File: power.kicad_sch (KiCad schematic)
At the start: 24 parts, among them J1 USB_C_Receptacle_USB2.0_14P, J8 Conn_01x04, J9 Conn_01x04, U4 TPS6282x

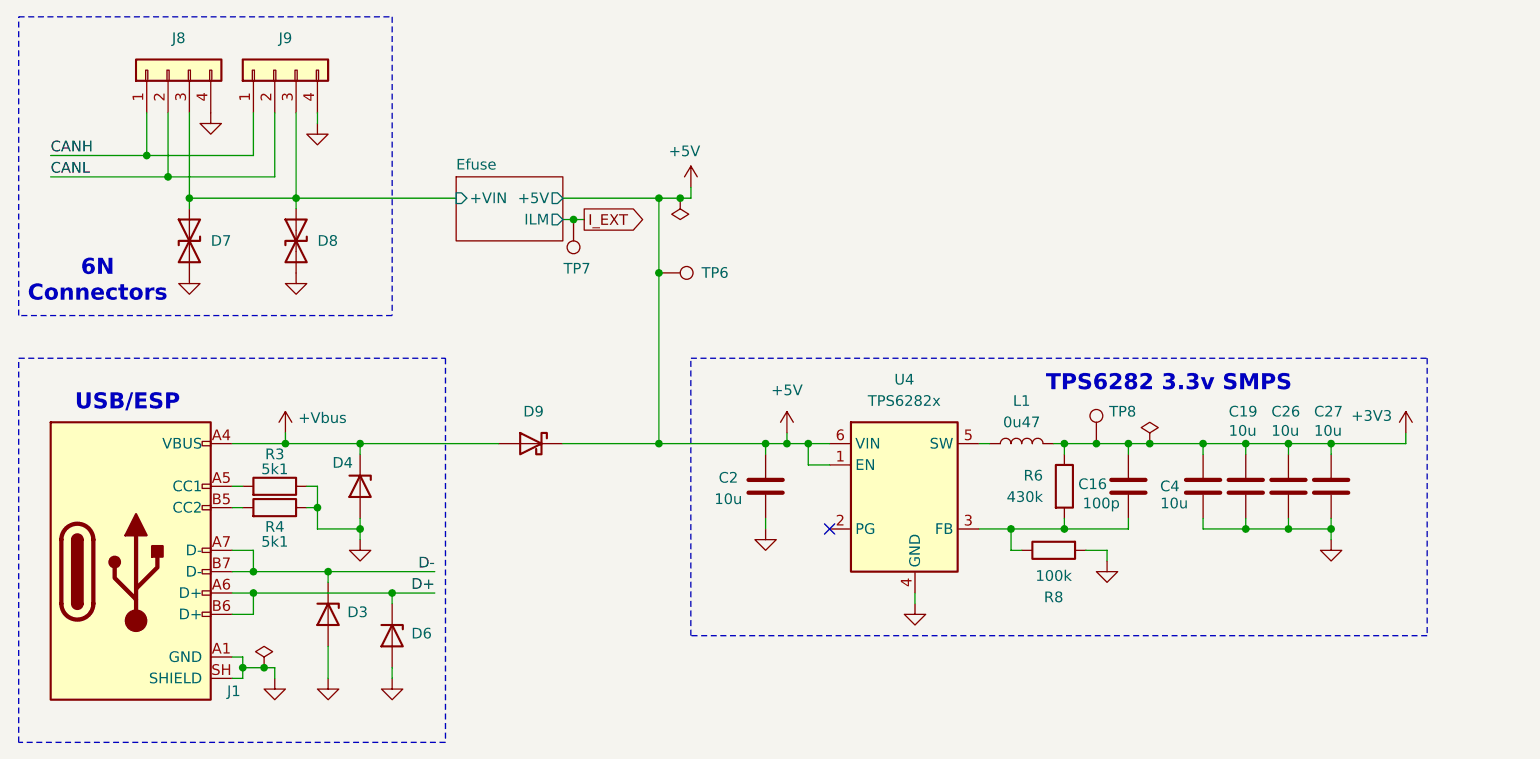
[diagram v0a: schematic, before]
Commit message: schem: add +3v8 smps
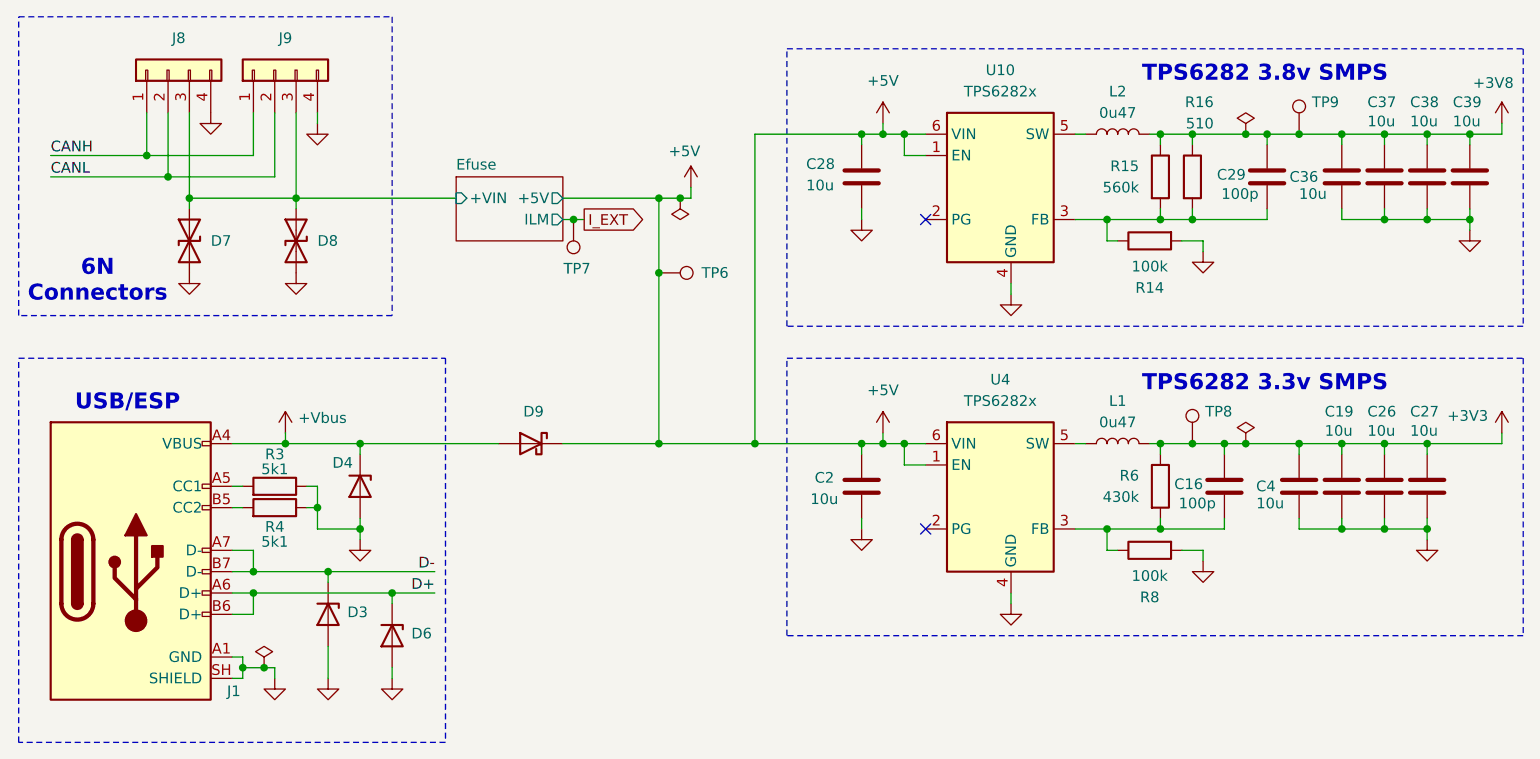
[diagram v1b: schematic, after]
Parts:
- added C28: 10u, Capacitor_SMD:C_0603_1608Metric, symbol Device:C
- added C29: 100p, Capacitor_SMD:C_0402_1005Metric, symbol Device:C
- added C36, C37, C38, C39: 10u, Capacitor_SMD:C_0402_1005Metric, symbol Device:C
- added L2: 0u47, Pers:TDK_TFM201610ALC, symbol Device:L
- added R14: 100k, Resistor_SMD:R_0402_1005Metric, symbol Device:R
- added R15: 560k, Resistor_SMD:R_0603_1608Metric, symbol Device:R
- added R16: 510, Resistor_SMD:R_0603_1608Metric, symbol Device:R
- added TP9: TestPoint, TestPoint:TestPoint_Pad_D2.0mm, symbol Connector:TestPoint
- added U10: TPS6282x, Pers:Texas_VSON-6_1.5x1.5mm_P0.5mm_DMQ0006A, symbol Pers:TPS6282x
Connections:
- net +5V: now also C28.1, U10.1 (EN), U10.6 (VIN)
- net GND: now also C28.2, C36.2, C37.2, C38.2, C39.2, R14.2, U10.4 (GND)
- new net: C29.2, R14.1, R15.2, R16.2, U10.3 (FB)
- new net: L2.1, U10.5 (SW)
- new net +3V8: C29.1, C36.1, C37.1, C38.1, C39.1, L2.2, R15.1, R16.1, TP9.1
- no-connect marks 1 -> 2
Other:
- note added: "TPS6282 3.8v SMPS"
- moved on the sheet: C16, C19, C2, C26, C27, C4, L1, R6, R8, TP8, U4
